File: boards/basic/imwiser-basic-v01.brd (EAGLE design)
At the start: 53 x 46 mm, 15 parts, among them J1-A3 PJ-313-SPAD, J2-A2 PJ-313-SPAD, J3-A1 PJ-313-SPAD, J4-D3 PJ-313-SPAD, J5-D5 PJ-313-SPAD, J6-D6 PJ-313-SPAD, U1 ARDUINO_SHIELDNO_SILK

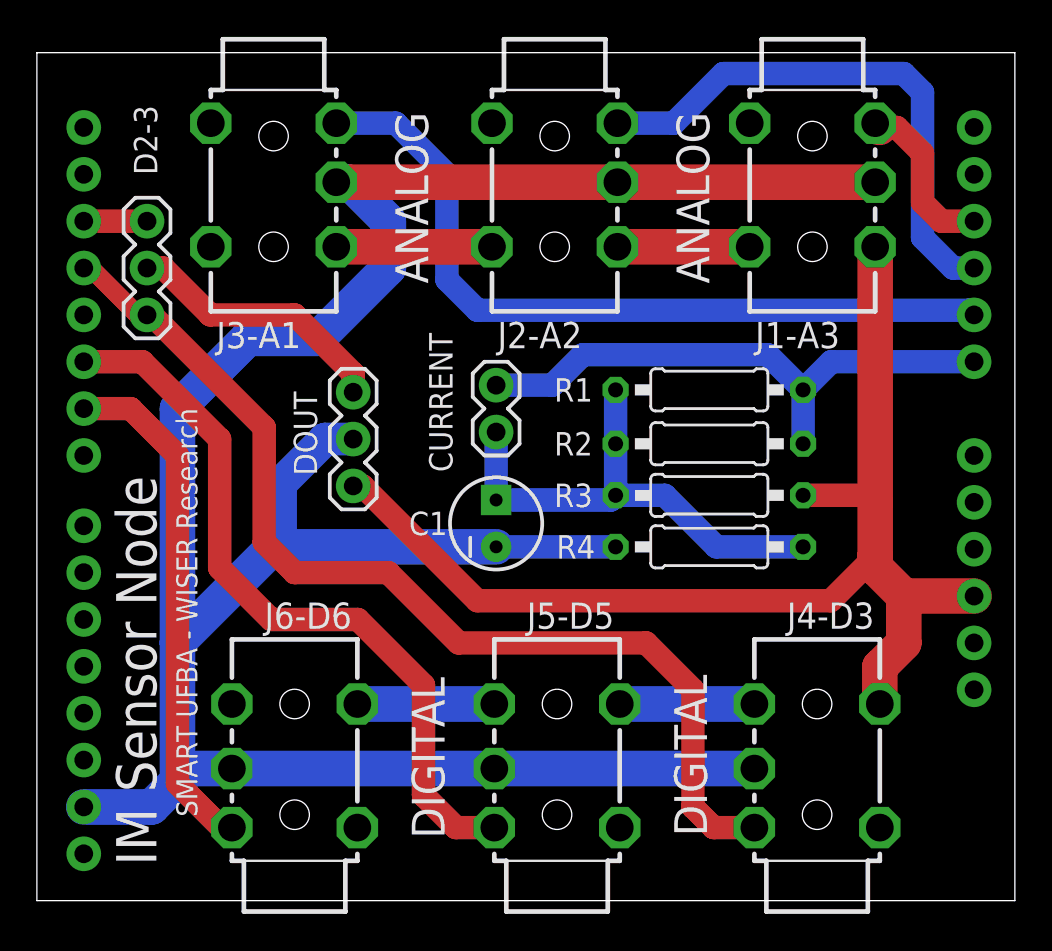
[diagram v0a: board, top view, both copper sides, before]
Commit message: Organized files, left organize cam jobs and libraries
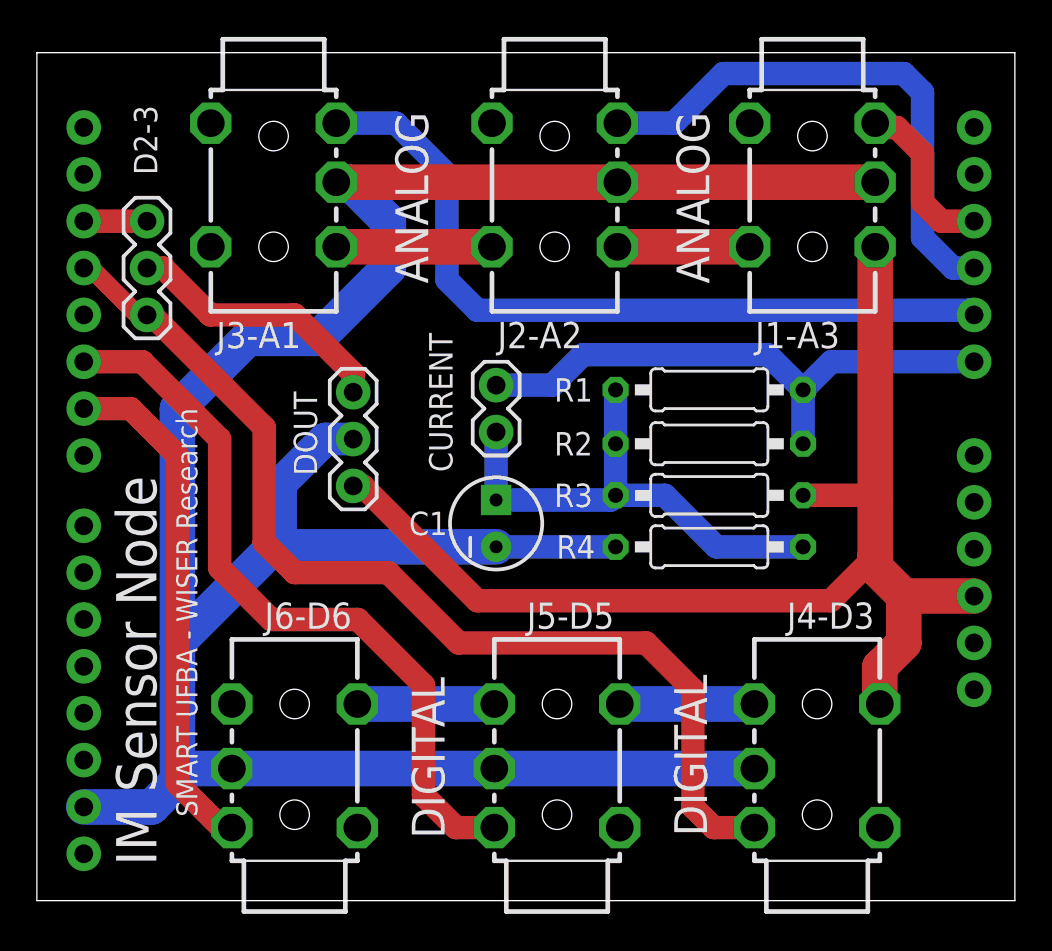
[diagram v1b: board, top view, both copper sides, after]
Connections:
- net J5 renamed D6
- net N$10 renamed A0
- net N$11 renamed BURDEN-C0
- net N$13 renamed D3
- net N$14 renamed D2
- net N$3 renamed A3
- net N$4 renamed A2
- net N$5 renamed A1
- net N$6 renamed D5
- net N$8 renamed OPTION-D2-3
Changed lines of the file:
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@@
 <layer number="230" name="230bmp" color="7" fill="1" visible="no" active="yes"/>
 <layer number="231" name="231bmp" color="7" fill="1" visible="no" active="yes"/>
+<layer number="232" name="Eagle3D_PG2" color="7" fill="1" visible="no" active="no"/>
+<layer number="233" name="Eagle3D_PG3" color="7" fill="1" visible="no" active="no"/>
 <layer number="248" name="Housing" color="7" fill="1" visible="no" active="yes"/>
 <layer number="249" name="Edge" color="7" fill="1" visible="no" active="yes"/>
@@
 </elements>
 <signals>
-<signal name="N$3">
-<contactref element="J1-A3" pad="1.1"/>
-<wire x1="45.669" y1="41.91" x2="45.437" y2="42.142" width="1.9304" layer="1"/>
+<signal name="A3">
 <contactref element="U1" pad="A3"/>
-<wire x1="45.669" y1="41.91" x2="46.609" y2="41.91" width="1.27" layer="1"/>
+<wire x1="45.437" y1="41.91" x2="46.609" y2="41.91" width="1.27" layer="1"/>
 <wire x1="46.609" y1="41.91" x2="48.006" y2="40.513" width="1.27" layer="1"/>
 <wire x1="48.006" y1="40.513" x2="48.006" y2="37.846" width="1.27" layer="1"/>
 <wire x1="48.006" y1="37.846" x2="49.022" y2="36.83" width="1.27" layer="1"/>
 <wire x1="49.022" y1="36.83" x2="50.8" y2="36.83" width="1.27" layer="1"/>
-</signal>
-<signal name="J5">
-<contactref element="U1" pad="D6"/>
+<contactref element="J1-A3" pad="1.1"/>
+<wire x1="45.437" y1="41.91" x2="45.437" y2="42.142" width="1.27" layer="1"/>
+</signal>
+<signal name="D6">
 <contactref element="J6-D6" pad="1.1"/>
 <wire x1="10.57" y1="3.959" x2="10.011" y2="3.959" width="1.27" layer="1"/>
@@
 <wire x1="7.62" y1="6.35" x2="7.62" y2="24.13" width="1.27" layer="1"/>
 <wire x1="7.62" y1="24.13" x2="5.08" y2="26.67" width="1.27" layer="1"/>
+<contactref element="U1" pad="D6"/>
 <wire x1="5.08" y1="26.67" x2="2.54" y2="26.67" width="1.27" layer="1"/>
 </signal>
@@
 <wire x1="24.667" y1="35.442" x2="16.227" y2="35.442" width="1.9304" layer="1"/>
 </signal>
-<signal name="N$5">
-<contactref element="J3-A1" pad="1.1"/>
+<signal name="A1">
 <wire x1="23.876" y1="32.004" x2="22.225" y2="33.655" width="1.27" layer="16"/>
 <wire x1="22.225" y1="33.655" x2="22.225" y2="39.37" width="1.27" layer="16"/>
 <wire x1="23.876" y1="32.004" x2="50.546" y2="32.004" width="1.27" layer="16"/>
-<wire x1="16.227" y1="42.142" x2="19.453" y2="42.142" width="1.27" layer="16"/>
 <wire x1="19.453" y1="42.142" x2="22.225" y2="39.37" width="1.27" layer="16"/>
 <contactref element="U1" pad="A1"/>
 <wire x1="50.546" y1="32.004" x2="50.8" y2="31.75" width="1.27" layer="16"/>
+<contactref element="J3-A1" pad="1.1"/>
+<wire x1="19.453" y1="42.142" x2="16.227" y2="42.142" width="1.27" layer="16"/>
 </signal>
 <signal name="GND">
@@
 <wire x1="38.891" y1="10.659" x2="31.594" y2="10.659" width="1.9304" layer="16"/>
 </signal>
-<signal name="N$6">
-<contactref element="U1" pad="D5"/>
+<signal name="D5">
 <contactref element="J5-D5" pad="1.1"/>
 <wire x1="24.794" y1="3.959" x2="22.711" y2="3.959" width="1.27" layer="1"/>
@@
 <wire x1="9.906" y1="18.034" x2="9.906" y2="25.019" width="1.27" layer="1"/>
 <wire x1="9.906" y1="25.019" x2="5.715" y2="29.21" width="1.27" layer="1"/>
+<wire x1="20.955" y1="11.684" x2="20.955" y2="5.715" width="1.27" layer="1"/>
+<contactref element="U1" pad="D5"/>
 <wire x1="5.715" y1="29.21" x2="2.54" y2="29.21" width="1.27" layer="1"/>
-<wire x1="20.955" y1="11.684" x2="20.955" y2="5.715" width="1.27" layer="1"/>
-</signal>
-<signal name="N$11">
+</signal>
+<signal name="BURDEN-C0">
 <contactref element="C1" pad="1"/>
 <contactref element="R1" pad="1"/>
@@
 <wire x1="24.892" y1="25.4" x2="24.892" y2="21.717" width="1.27" layer="16"/>
 </signal>
-<signal name="N$10">
+<signal name="A0">
 <contactref element="R2" pad="2"/>
 <contactref element="R1" pad="2"/>
-<contactref element="U1" pad="A0"/>
 <wire x1="41.529" y1="24.765" x2="41.529" y2="27.686" width="1.27" layer="16"/>
-<wire x1="50.8" y1="29.21" x2="43.053" y2="29.21" width="1.27" layer="16"/>
 <wire x1="43.053" y1="29.21" x2="41.529" y2="27.686" width="1.27" layer="16"/>
 <contactref element="CURRENT" pad="2"/>
@@
 <wire x1="27.94" y1="27.94" x2="29.591" y2="29.591" width="1.27" layer="16"/>
 <wire x1="24.892" y1="27.94" x2="27.94" y2="27.94" width="1.27" layer="16"/>
-</signal>
-<signal name="N$4">
+<contactref element="U1" pad="A0"/>
+<wire x1="43.053" y1="29.21" x2="50.8" y2="29.21" width="1.27" layer="16"/>
+</signal>
+<signal name="A2">
 <contactref element="U1" pad="A2"/>
-<contactref element="J2-A2" pad="1.1"/>
-<wire x1="31.467" y1="42.142" x2="34.522" y2="42.142" width="1.27" layer="16"/>
 <wire x1="34.522" y1="42.142" x2="37.211" y2="44.831" width="1.27" layer="16"/>
 <wire x1="37.211" y1="44.831" x2="46.99" y2="44.831" width="1.27" layer="16"/>
@@
 <wire x1="48.006" y1="35.941" x2="49.657" y2="34.29" width="1.27" layer="16"/>
 <wire x1="49.657" y1="34.29" x2="50.8" y2="34.29" width="1.27" layer="16"/>
-</signal>
-<signal name="N$14">
+<contactref element="J2-A2" pad="1.1"/>
+<wire x1="34.522" y1="42.142" x2="31.467" y2="42.142" width="1.27" layer="16"/>
+</signal>
+<signal name="D2">
 <contactref element="D2-3" pad="3"/>
 <contactref element="U1" pad="D2"/>
 <wire x1="5.969" y1="36.83" x2="2.54" y2="36.83" width="1.27" layer="1"/>
 </signal>
-<signal name="N$13">
+<signal name="D3">
 <contactref element="J4-D3" pad="1.1"/>
 <wire x1="38.891" y1="3.959" x2="36.681" y2="3.959" width="1.27" layer="1"/>
@@
 <wire x1="13.97" y1="17.78" x2="12.319" y2="19.431" width="1.27" layer="1"/>
 <wire x1="12.319" y1="19.431" x2="12.319" y2="25.654" width="1.27" layer="1"/>
+<wire x1="6.223" y1="31.75" x2="12.319" y2="25.654" width="1.27" layer="1"/>
 <contactref element="U1" pad="D3"/>
 <contactref element="D2-3" pad="1"/>
@@
 <wire x1="2.921" y1="34.29" x2="5.461" y2="31.75" width="1.016" layer="1"/>
 <wire x1="5.461" y1="31.75" x2="5.969" y2="31.75" width="1.016" layer="1"/>
-<wire x1="5.969" y1="31.75" x2="6.223" y2="31.75" width="1.27" layer="1"/>
-<wire x1="6.223" y1="31.75" x2="12.319" y2="25.654" width="1.27" layer="1"/>
-</signal>
-<signal name="N$8">
+<wire x1="6.223" y1="31.75" x2="5.969" y2="31.75" width="1.27" layer="1"/>
+</signal>
+<signal name="OPTION-D2-3">
 <contactref element="DOUT" pad="3"/>
 <contactref element="D2-3" pad="2"/>
